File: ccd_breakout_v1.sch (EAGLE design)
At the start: 9 parts, among them IC2 74AS04D

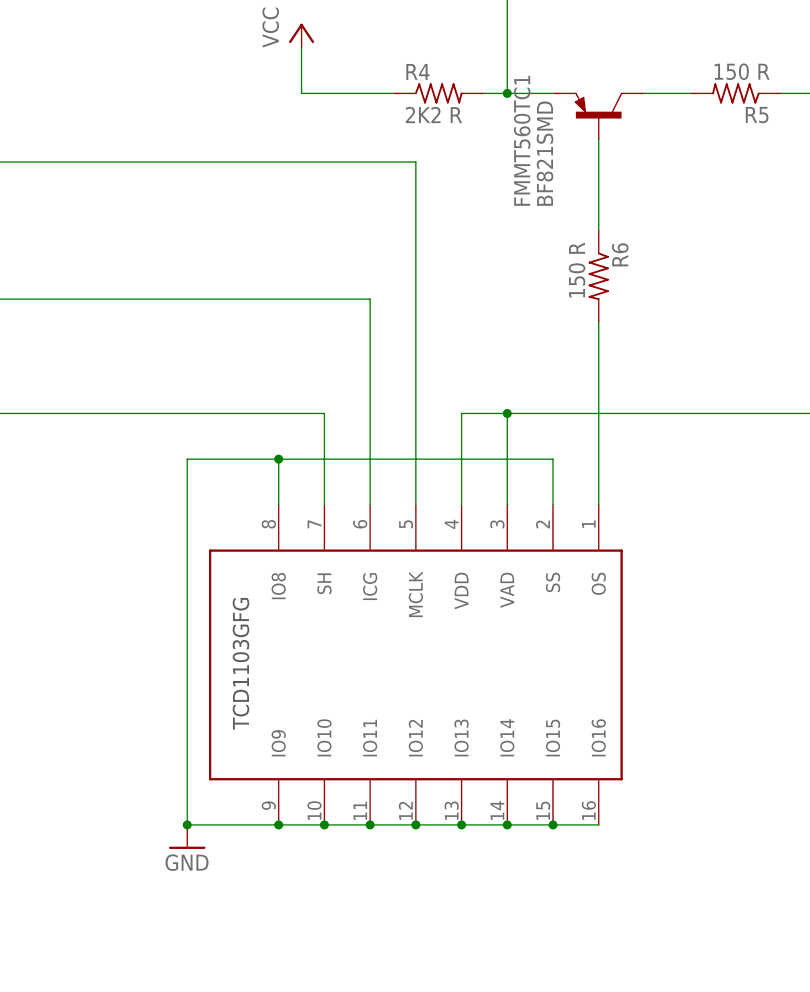
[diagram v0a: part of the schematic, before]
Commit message: ccdDone
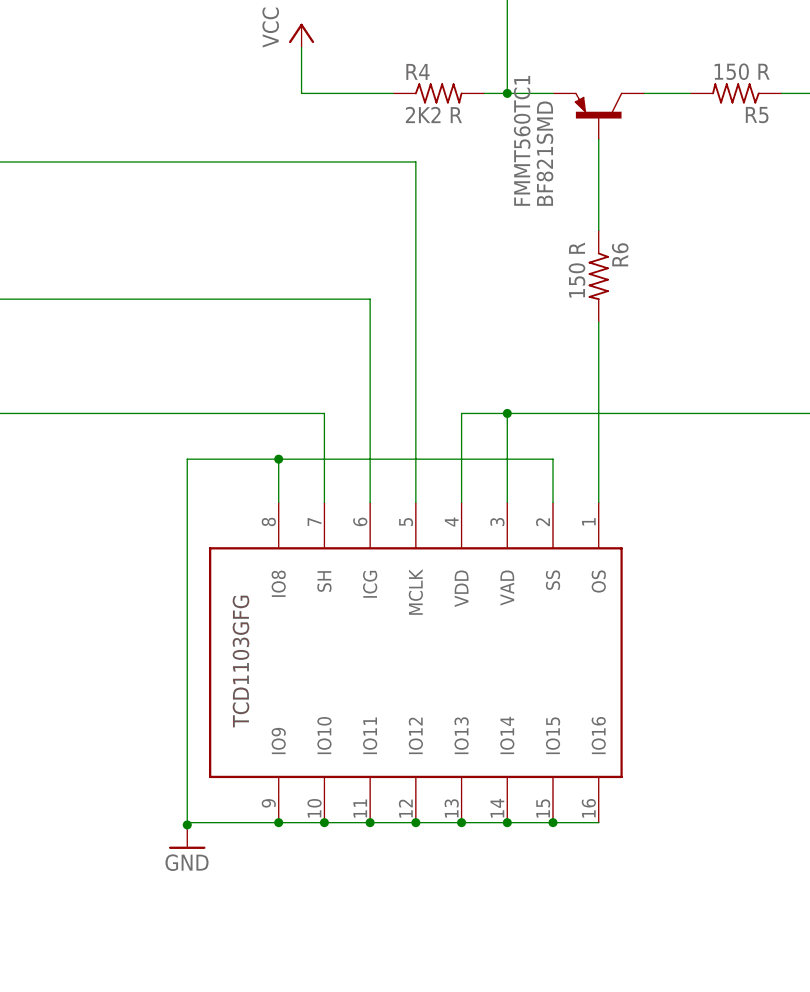
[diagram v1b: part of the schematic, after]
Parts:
- removed U$2: TCD1103, TCD1103:TCD1103
- added U$1: TCD1103_TCD1103, spectrometer_mother_board_v1:TCD1103_TCD1103
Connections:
- net GND: now also U$1.IO10, U$1.IO11, U$1.IO12, U$1.IO13, U$1.IO14, U$1.IO15, U$1.IO16, U$1.IO8, U$1.IO9, U$1.SS; no longer U$2.IO10, U$2.IO11, U$2.IO12, U$2.IO13, U$2.IO14, U$2.IO15, U$2.IO16, U$2.IO8, U$2.IO9, U$2.SS
- net N$10: now also U$1.MCLK; no longer U$2.MCLK
- net N$11: now also U$1.ICG; no longer U$2.ICG
- net N$12: now also U$1.SH; no longer U$2.SH
- net N$9: now also U$1.OS; no longer U$2.OS
- net VCC: now also U$1.VAD, U$1.VDD; no longer U$2.VAD, U$2.VDD
